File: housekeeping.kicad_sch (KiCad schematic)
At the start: 8 parts, among them U5 TPS7B8133QDGNRQ1

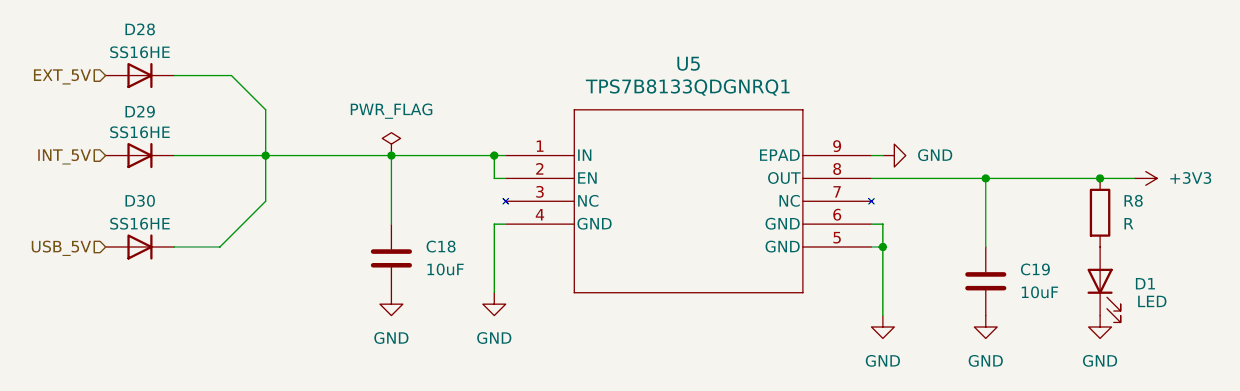
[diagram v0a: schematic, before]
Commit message: prepaing for production
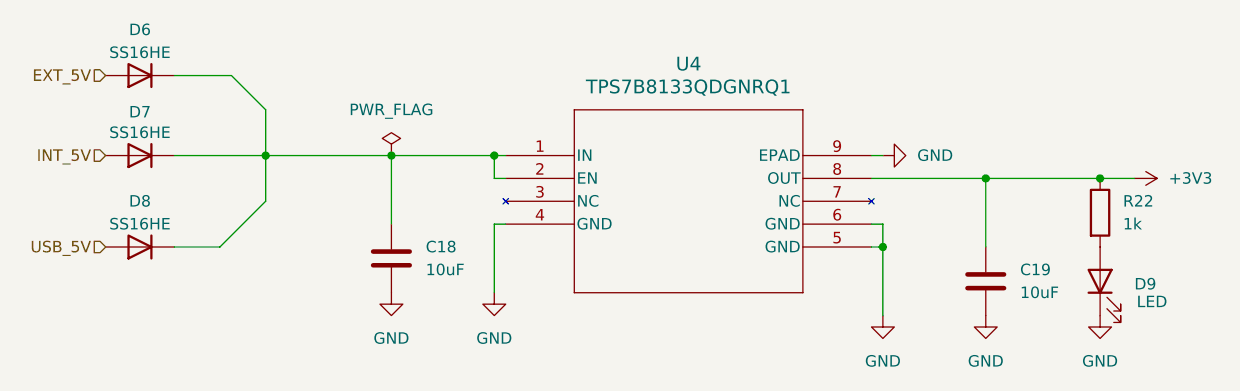
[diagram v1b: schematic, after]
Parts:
- C18, C19: Supplier_2 (none) -> JLCPCB; Supplier_2 P/N (none) -> C440198
- D6: renamed from D28; Supplier_2 (none) -> JLCPCB; Supplier_2 P/N (none) -> C556433
- D7: renamed from D29; Supplier_2 (none) -> JLCPCB; Supplier_2 P/N (none) -> C556433
- D8: renamed from D30; Supplier_2 (none) -> JLCPCB; Supplier_2 P/N (none) -> C556433
- D9: renamed from D1; Mfr (none) -> ROHM Semi; Mfr P/N (none) -> SML-E12P8WT86; Supplier_2 (none) -> JLCPCB; Supplier_2 P/N (none) -> C126319
- R22: renamed from R8; value R -> 1k; Mfr (none) -> YAGEO; Mfr P/N (none) -> AC0603FR-071KL; Supplier_2 (none) -> JLCPCB; Supplier_2 P/N (none) -> C116692
- renumbered U5 to U4
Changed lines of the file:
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@@
 		(dnp no)
 		(fields_autoplaced yes)
-		(property "Reference" "#PWR067"
+		(property "Reference" "#PWR065"
 			(at 193.04 123.19 0)
 			(effects
@@
 			(project "BMS"
 				(path "/124184ba-5d68-4d9f-8da6-acc6720ab30b/93f9b420-7cce-46a9-9201-666f07a18f85/1875dae8-5675-4324-bc32-eabf0e306a05"
-					(reference "#PWR067")
+					(reference "#PWR065")
 					(unit 1)
 				)
@@
 		(dnp no)
 		(fields_autoplaced yes)
-		(property "Reference" "#PWR068"
+		(property "Reference" "#PWR066"
 			(at 193.04 101.6 0)
 			(effects
@@
 			(project "BMS"
 				(path "/124184ba-5d68-4d9f-8da6-acc6720ab30b/93f9b420-7cce-46a9-9201-666f07a18f85/1875dae8-5675-4324-bc32-eabf0e306a05"
-					(reference "#PWR068")
+					(reference "#PWR066")
 					(unit 1)
 				)
@@
 		(dnp no)
 		(fields_autoplaced yes)
-		(property "Reference" "#FLG03"
+		(property "Reference" "#FLG04"
 			(at 114.3 97.155 0)
 			(effects
@@
 			(project ""
 				(path "/124184ba-5d68-4d9f-8da6-acc6720ab30b/93f9b420-7cce-46a9-9201-666f07a18f85/1875dae8-5675-4324-bc32-eabf0e306a05"
-					(reference "#FLG03")
+					(reference "#FLG04")
 					(unit 1)
 				)
@@
 		(dnp no)
 		(fields_autoplaced yes)
-		(property "Reference" "#PWR064"
+		(property "Reference" "#PWR062"
 			(at 175.26 99.06 0)
 			(effects
@@
 			(project "BMS"
 				(path "/124184ba-5d68-4d9f-8da6-acc6720ab30b/93f9b420-7cce-46a9-9201-666f07a18f85/1875dae8-5675-4324-bc32-eabf0e306a05"
-					(reference "#PWR064")
+					(reference "#PWR062")
 					(unit 1)
 				)
@@
 		(dnp no)
 		(fields_autoplaced yes)
-		(property "Reference" "#PWR062"
+		(property "Reference" "#PWR060"
 			(at 114.3 120.65 0)
 			(effects
@@
 			(project ""
 				(path "/124184ba-5d68-4d9f-8da6-acc6720ab30b/93f9b420-7cce-46a9-9201-666f07a18f85/1875dae8-5675-4324-bc32-eabf0e306a05"
-					(reference "#PWR062")
+					(reference "#PWR060")
 					(unit 1)
 				)
@@
 		(dnp no)
 		(fields_autoplaced yes)
-		(property "Reference" "R8"
+		(property "Reference" "R22"
 			(at 195.58 104.1399 0)
 			(effects
@@
 			)
 		)
-		(property "Value" "R"
+		(property "Value" "1k"
 			(at 195.58 106.6799 0)
 			(effects
@@
 			)
 		)
-		(property "Description" "Resistor"
+		(property "Description" "100mW 1kΩ 75V Thick Film Resistor ±1% ±100ppm/℃ 0603"
 			(at 193.04 105.41 0)
 			(effects
@@
 			)
 		)
-		(property "Mfr" ""
+		(property "Mfr" "YAGEO"
 			(at 193.04 105.41 0)
 			(effects
@@
 			)
 		)
-		(property "Mfr P/N" ""
+		(property "Mfr P/N" "AC0603FR-071KL"
 			(at 193.04 105.41 0)
 			(effects
@@
 			)
 		)
-		(property "Supplier_2" ""
+		(property "Supplier_2" "JLCPCB"
 			(at 193.04 105.41 0)
 			(effects
@@
 			)
 		)
-		(property "Supplier_2 P/N" ""
+		(property "Supplier_2 P/N" "C116692"
 			(at 193.04 105.41 0)
 			(effects
@@
 		)
 		(property "Supplier_2 Price @ Qty" ""
+			(at 193.04 105.41 0)
+			(effects
+				(font
+					(size 1.27 1.27)
+				)
+				(hide yes)
+			)
+		)
+		(property "DigiKey_Part_Number" ""
 			(at 193.04 105.41 0)
 			(effects
@@
 			(project "BMS"
 				(path "/124184ba-5d68-4d9f-8da6-acc6720ab30b/93f9b420-7cce-46a9-9201-666f07a18f85/1875dae8-5675-4324-bc32-eabf0e306a05"
-					(reference "R8")
+					(reference "R22")
 					(unit 1)
 				)
@@
 		(dnp no)
 		(fields_autoplaced yes)
-		(property "Reference" "U5"
+		(property "Reference" "U4"
 			(at 147.32 88.9 0)
 			(effects
@@
 		)
 		(property "Supplier_2 Price @ Qty" "1"
+			(at 127 99.06 0)
+			(effects
+				(font
+					(size 1.27 1.27)
+				)
+				(hide yes)
+			)
+		)
+		(property "DigiKey_Part_Number" ""
 			(at 127 99.06 0)
 			(effects
@@
 			(project ""
 				(path "/124184ba-5d68-4d9f-8da6-acc6720ab30b/93f9b420-7cce-46a9-9201-666f07a18f85/1875dae8-5675-4324-bc32-eabf0e306a05"
-					(reference "U5")
+					(reference "U4")
 					(unit 1)
 				)
@@
 		(on_board yes)
 		(dnp no)
-		(property "Reference" "D28"
+		(property "Reference" "D6"
 			(at 86.36 85.09 0)
 			(effects
@@
 			)
 		)
-		(property "Supplier_2" ""
+		(property "Supplier_2" "JLCPCB"
 			(at 86.36 90.17 0)
 			(effects
@@
 			)
 		)
-		(property "Supplier_2 P/N" ""
+		(property "Supplier_2 P/N" "C556433"
 			(at 86.36 90.17 0)
 			(effects
@@
 		)
 		(property "Supplier_2 Price @ Qty" ""
+			(at 86.36 90.17 0)
+			(effects
+				(font
+					(size 1.27 1.27)
+				)
+				(hide yes)
+			)
+		)
+		(property "DigiKey_Part_Number" ""
 			(at 86.36 90.17 0)
 			(effects
@@
 			(project "BMS"
 				(path "/124184ba-5d68-4d9f-8da6-acc6720ab30b/93f9b420-7cce-46a9-9201-666f07a18f85/1875dae8-5675-4324-bc32-eabf0e306a05"
-					(reference "D28")
+					(reference "D6")
 					(unit 1)
 				)
@@
 		(on_board yes)
 		(dnp no)
-		(property "Reference" "D30"
+		(property "Reference" "D8"
 			(at 86.36 104.14 0)
 			(effects
@@
 			)
 		)
-		(property "Supplier_2" ""
+		(property "Supplier_2" "JLCPCB"
 			(at 86.36 109.22 0)
 			(effects
@@
 			)
 		)
-		(property "Supplier_2 P/N" ""
+		(property "Supplier_2 P/N" "C556433"
 			(at 86.36 109.22 0)
 			(effects
@@
 		)
 		(property "Supplier_2 Price @ Qty" ""
+			(at 86.36 109.22 0)
+			(effects
+				(font
+					(size 1.27 1.27)
+				)
+				(hide yes)
+			)
+		)
+		(property "DigiKey_Part_Number" ""
 			(at 86.36 109.22 0)
 			(effects
@@
 			(project "BMS"
 				(path "/124184ba-5d68-4d9f-8da6-acc6720ab30b/93f9b420-7cce-46a9-9201-666f07a18f85/1875dae8-5675-4324-bc32-eabf0e306a05"
-					(reference "D30")
+					(reference "D8")
 					(unit 1)
 				)
@@
 		(dnp no)
 		(fields_autoplaced yes)
-		(property "Reference" "#PWR063"
+		(property "Reference" "#PWR061"
 			(at 125.73 120.65 0)
 			(effects
@@
 			(project "BMS"
 				(path "/124184ba-5d68-4d9f-8da6-acc6720ab30b/93f9b420-7cce-46a9-9201-666f07a18f85/1875dae8-5675-4324-bc32-eabf0e306a05"
-					(reference "#PWR063")
+					(reference "#PWR061")
 					(unit 1)
 				)
@@
 			)
 		)
-		(property "Supplier_2" ""
+		(property "Supplier_2" "JLCPCB"
 			(at 114.3 110.49 0)
 			(effects
@@
 			)
 		)
-		(property "Supplier_2 P/N" ""
+		(property "Supplier_2 P/N" "C440198"
 			(at 114.3 110.49 0)
 			(effects
@@
 		)
 		(property "Supplier_2 Unit Price" ""
+			(at 114.3 110.49 0)
+			(effects
+				(font
+					(size 1.27 1.27)
+				)
+				(hide yes)
+			)
+		)
+		(property "DigiKey_Part_Number" ""
 			(at 114.3 110.49 0)
 			(effects
@@
 		(dnp no)
 		(fields_autoplaced yes)
-		(property "Reference" "#PWR066"
+		(property "Reference" "#PWR064"
 			(at 180.34 123.19 0)
 			(effects
@@
 			(project "BMS"
 				(path "/124184ba-5d68-4d9f-8da6-acc6720ab30b/93f9b420-7cce-46a9-9201-666f07a18f85/1875dae8-5675-4324-bc32-eabf0e306a05"
-					(reference "#PWR066")
+					(reference "#PWR064")
 					(unit 1)
 				)
@@
 			)
 		)
-		(property "Supplier_2" ""
+		(property "Supplier_2" "JLCPCB"
 			(at 180.34 113.03 0)
 			(effects
@@
 			)
 		)
-		(property "Supplier_2 P/N" ""
+		(property "Supplier_2 P/N" "C440198"
 			(at 180.34 113.03 0)
 			(effects
@@
 		)
 		(property "Supplier_2 Unit Price" ""
+			(at 180.34 113.03 0)
+			(effects
+				(font
+					(size 1.27 1.27)
+				)
+				(hide yes)
+			)
+		)
+		(property "DigiKey_Part_Number" ""
 			(at 180.34 113.03 0)
 			(effects
@@
 		(dnp no)
 		(fields_autoplaced yes)
-		(property "Reference" "#PWR065"
+		(property "Reference" "#PWR063"
 			(at 168.91 123.19 0)
 			(effects
@@
 			(project "BMS"
 				(path "/124184ba-5d68-4d9f-8da6-acc6720ab30b/93f9b420-7cce-46a9-9201-666f07a18f85/1875dae8-5675-4324-bc32-eabf0e306a05"
-					(reference "#PWR065")
+					(reference "#PWR063")
 					(unit 1)
 				)
@@
 		(on_board yes)
 		(dnp no)
-		(property "Reference" "D1"
+		(property "Reference" "D9"
 			(at 196.85 113.3474 90)
 			(effects
@@
 			)
 		)
-		(property "Description" "Light emitting diode"
+		(property "Description" ".2V 20mA 54mW 560nm 6.3mcd Common Cathode Green White"
 			(at 193.04 113.03 0)
 			(effects
@@
 			)
 		)
-		(property "Mfr" ""
+		(property "Mfr" "ROHM Semi"
 			(at 193.04 113.03 0)
 			(effects
@@
 			)
 		)
-		(property "Mfr P/N" ""
+		(property "Mfr P/N" "SML-E12P8WT86"
 			(at 193.04 113.03 0)
 			(effects
@@
 			)
 		)
-		(property "Supplier_2" ""
+		(property "Supplier_2" "JLCPCB"
 			(at 193.04 113.03 0)
 			(effects
@@
 			)
 		)
-		(property "Supplier_2 P/N" ""
+		(property "Supplier_2 P/N" "C126319"
 			(at 193.04 113.03 0)
 			(effects
@@
 		(property "Supplier_2 Price @ Qty" ""
 			(at 193.04 113.03 0)
+			(effects
+				(font
+					(size 1.27 1.27)
+				)
+				(hide yes)
+			)
+		)
+		(property "DigiKey_Part_Number" ""
+			(at 193.04 113.03 90)
 			(effects
 				(font
@@
 			(project "BMS"
 				(path "/124184ba-5d68-4d9f-8da6-acc6720ab30b/93f9b420-7cce-46a9-9201-666f07a18f85/1875dae8-5675-4324-bc32-eabf0e306a05"
-					(reference "D1")
+					(reference "D9")
 					(unit 1)
 				)
@@
 		(on_board yes)
 		(dnp no)
-		(property "Reference" "D29"
+		(property "Reference" "D7"
 			(at 86.36 94.234 0)
 			(effects
@@
 			)
 		)
-		(property "Supplier_2" ""
+		(property "Supplier_2" "JLCPCB"
 			(at 86.36 99.06 0)
 			(effects
@@
 			)
 		)
-		(property "Supplier_2 P/N" ""
+		(property "Supplier_2 P/N" "C556433"
 			(at 86.36 99.06 0)
 			(effects
@@
 		)
 		(property "Supplier_2 Price @ Qty" ""
+			(at 86.36 99.06 0)
+			(effects
+				(font
+					(size 1.27 1.27)
+				)
+				(hide yes)
+			)
+		)
+		(property "DigiKey_Part_Number" ""
 			(at 86.36 99.06 0)
 			(effects
@@
 			(project "BMS"
 				(path "/124184ba-5d68-4d9f-8da6-acc6720ab30b/93f9b420-7cce-46a9-9201-666f07a18f85/1875dae8-5675-4324-bc32-eabf0e306a05"
-					(reference "D29")
+					(reference "D7")
 					(unit 1)
 				)
